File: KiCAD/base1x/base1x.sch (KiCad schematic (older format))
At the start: 82 parts, among them J1 Conn_02x05_Odd_Even, J10 Conn_01x03, J11 Conn_01x03, J12 Conn_01x03, J13 Conn_01x03, J14 Conn_01x03, J15 Conn_01x08, J17 Conn_01x03, J18 Conn_01x03, J19 Conn_01x03, J2 Conn_01x03, J3 Conn_02x14_Counter_Clockwise, J4 Conn_01x03, J5 Conn_01x03, J6 Conn_02x14_Counter_Clockwise, J7 Conn_02x06_Counter_Clockwise, J8 Conn_02x06_Counter_Clockwise, J9 Screw_Terminal_01x08, U2 ads122c04, U3 AD8615, U5 ads122c04, U6 AD8615, U7 AD8615, U8 LT1963AxQ-2.5, U9 LT3015xQ-2.5

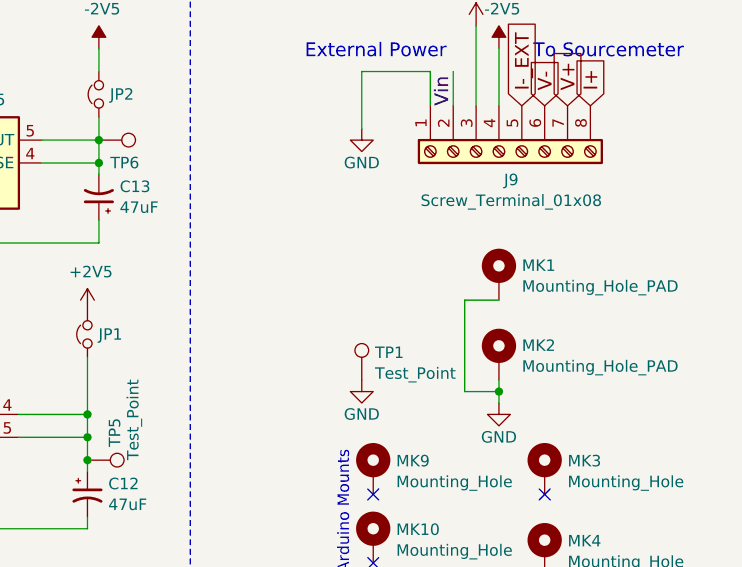
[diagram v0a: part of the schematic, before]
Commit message: work sync
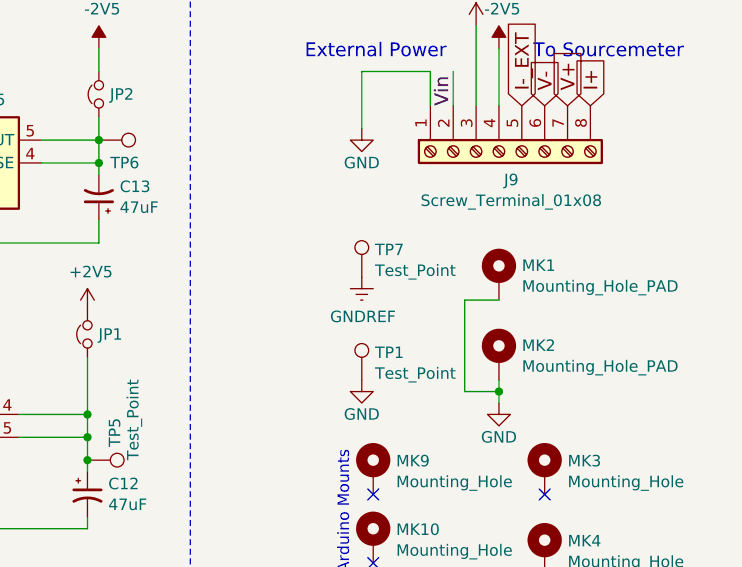
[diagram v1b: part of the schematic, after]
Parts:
- added TP7: Test_Point, myParts:Test_Point_S1751-46R, symbol Connector:TestPoint
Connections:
- net GNDREF: now also TP7.1
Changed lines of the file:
@@
 NoConn ~ 950  7400
 NoConn ~ 950  6900
+$Comp
+L Connector:TestPoint TP7
+U 1 1 5C3E8296
+P 9750 1850
+F 0 "TP7" H 9808 1970 50  0000 L CNN
+F 1 "Test_Point" H 9808 1879 50  0000 L CNN
+F 2 "myParts:Test_Point_S1751-46R" H 9950 1850 50  0001 C CNN
+F 3 "" H 9950 1850 50  0001 C CNN
+F 4 "2293786" H 4100 -4450 50  0001 C CNN "farnellCode"
+	1    9750 1850
+	1    0    0    -1
+$EndComp
+$Comp
+L power:GNDREF #PWR022
+U 1 1 5C3F39DD
+P 9750 1850
+F 0 "#PWR022" H 9750 1600 50  0001 C CNN
+F 1 "GNDREF" H 9755 1677 50  0000 C CNN
+F 2 "" H 9750 1850 50  0001 C CNN
+F 3 "" H 9750 1850 50  0001 C CNN
+	1    9750 1850
+	1    0    0    -1
+$EndComp
 $EndSCHEMATC

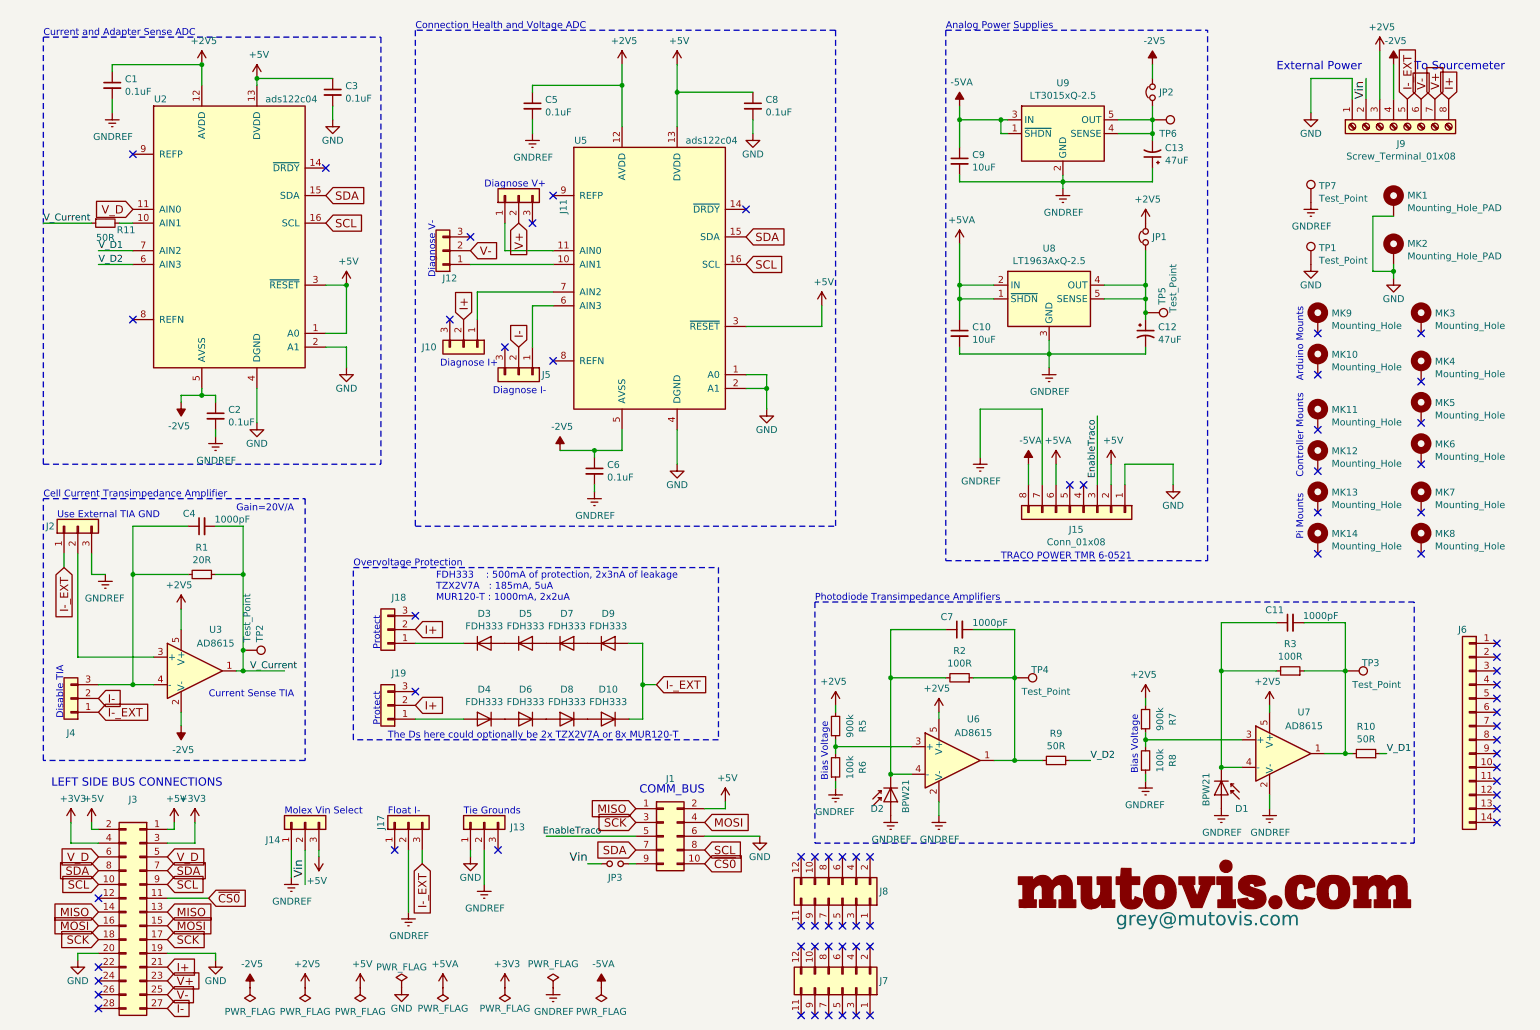
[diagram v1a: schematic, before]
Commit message: base1x doneish
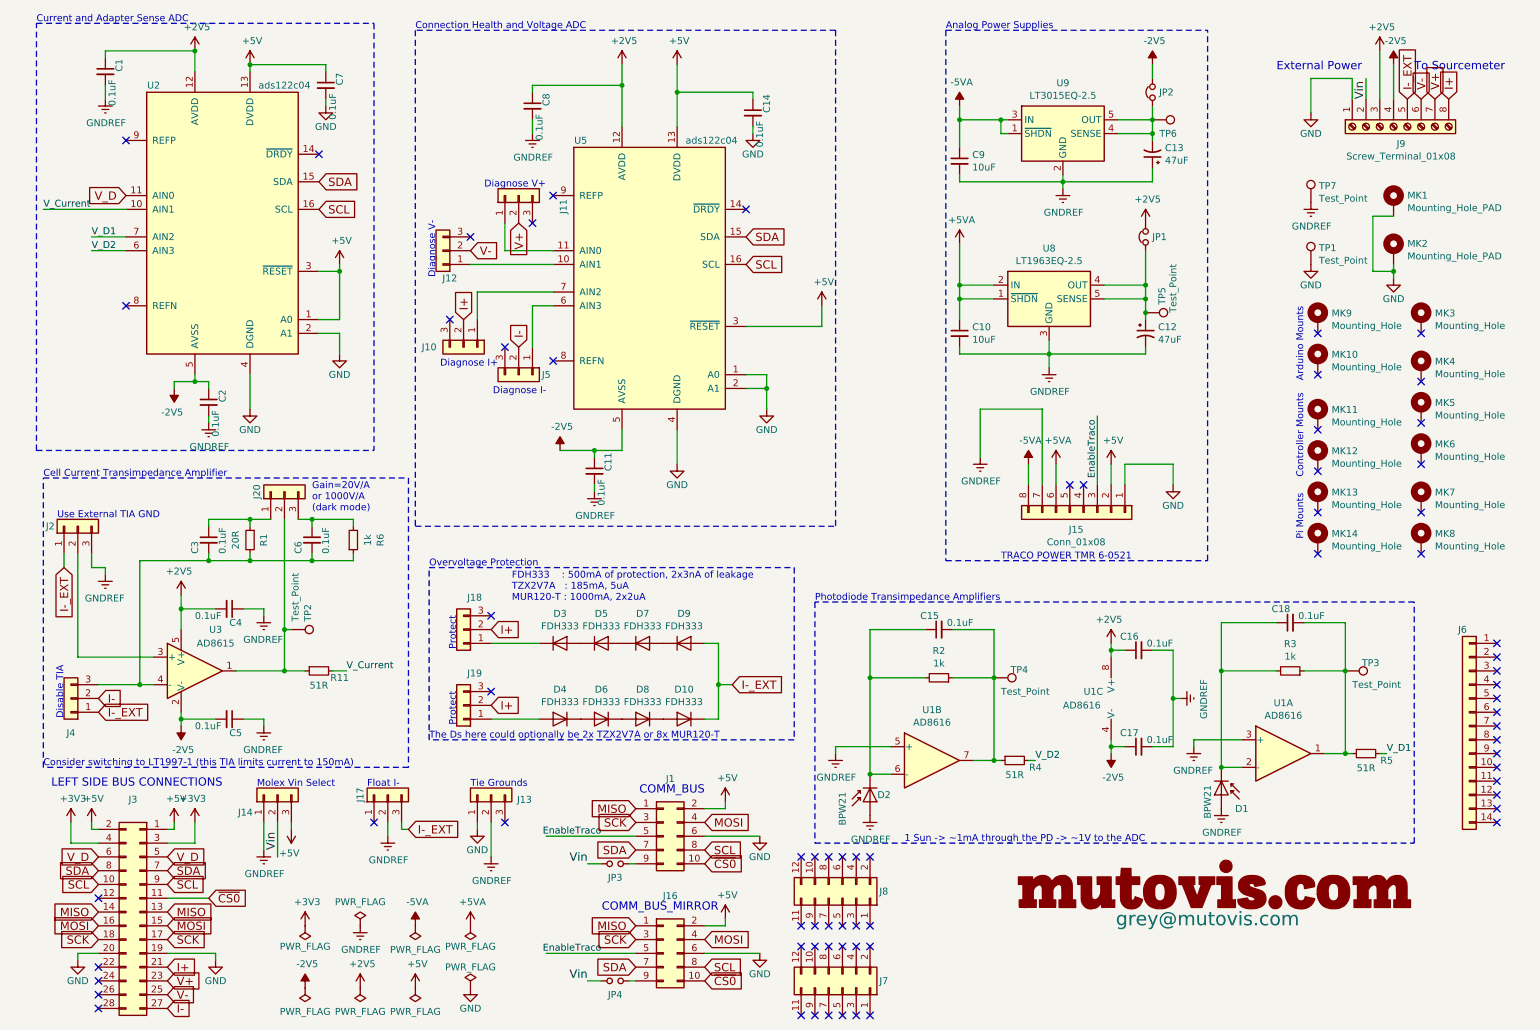
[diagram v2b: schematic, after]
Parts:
- removed R10, R9: 50R, Resistor_SMD:R_1206_3216Metric, symbol Device:R_Small
- removed R7: 900k, Resistor_SMD:R_1206_3216Metric, symbol Device:R_Small
- removed R8: 100k, Resistor_SMD:R_1206_3216Metric, symbol Device:R_Small
- removed U6, U7: AD8615, Package_TO_SOT_SMD:TSOT-23-5, symbol Amplifier_Operational:AD8603
- added C14, C15, C16, C17, C18: 0.1uF, Capacitor_SMD:C_1206_3216Metric, symbol Device:C_Small
- added J16: Conn_02x05_Odd_Even, Connector_IDC:IDC-Header_2x05_P2.54mm_Vertical, symbol Connector_Generic:Conn_02x05_Odd_Even
- added J20: Conn_01x03, Connector_PinHeader_1.27mm:PinHeader_1x03_P1.27mm_Vertical, symbol Connector_Generic:Conn_01x03
- added JP4: Jumper_NO_Small, Jumper:SolderJumper-2_P1.3mm_Open_RoundedPad1.0x1.5mm, symbol Device:Jumper_NO_Small
- added R4: 51R, Resistor_SMD:R_1206_3216Metric_Pad1.42x1.75mm_HandSolder, symbol Device:R_Small
- added U1: AD8616, Package_SO:SOIC-8_3.9x4.9mm_P1.27mm, symbol Amplifier_Operational:AD8620
- C1, C2, C3, C5, C6, C8: farnell code (none) -> 1759297
- C10, C9: farnell code (none) -> 1759453
- C11, C4, C7: value 1000pF -> 0.1uF; farnell code 1855909 -> 1759297
- C12, C13: footprint (none) -> Capacitor_Tantalum_SMD:CP_EIA-7343-43_Kemet-X_Pad2.25x2.55mm_HandSolder
- D1, D2: I_max 20mA -> 2mA
- D10, D3, D4, D5, D6, D7, D8, D9: farnellCode (none) -> 9843760
- J1: footprint Connector_IDC:IDC-Header_2x05_P2.54mm_Horizontal -> Connector_IDC:IDC-Header_2x05_P2.54mm_Vertical; farnellCode 2215290 -> 2215304
- J10, J11, J12, J13, J14, J17, J18, J19, J2, J4, J5: footprint (none) -> Connector_PinHeader_1.27mm:PinHeader_1x03_P1.27mm_Vertical; farnell code (none) -> 2578712+2505013
- J15: footprint (none) -> Converter_DCDC:Converter_DCDC_TRACO_TMR-xxxx_THT; Farnell Code (none) -> 495-TMR6-0521
- J3: farnell code (none) -> 1097986
- J6: value Conn_02x14_Counter_Clockwise -> Conn_01x14_Counter_Clockwise; footprint Connector_PinSocket_2.54mm:PinSocket_2x14_P2.54mm_Vertical -> Connector_PinHeader_2.54mm:PinHeader_1x14_P2.54mm_Vertical; farnellCode (none) -> 1593466
- JP3: footprint (none) -> Jumper:SolderJumper-2_P1.3mm_Open_RoundedPad1.0x1.5mm
- R1: footprint Resistor_SMD:R_1206_3216Metric -> Resistor_SMD:R_2010_5025Metric_Pad1.52x2.65mm_HandSolder; farnellCode 2073607 -> 1887405
- R11: value 50R -> 51R; footprint Resistor_SMD:R_1206_3216Metric -> Resistor_SMD:R_1206_3216Metric_Pad1.42x1.75mm_HandSolder; farnellCode 2476379 -> 2695165
- R2, R3: value 100R -> 1k; footprint Resistor_SMD:R_1206_3216Metric -> Resistor_SMD:R_1206_3216Metric_Pad1.42x1.75mm_HandSolder; farnellCode 2476379 -> 2447473
- R5: value 900k -> 51R; footprint Resistor_SMD:R_1206_3216Metric -> Resistor_SMD:R_1206_3216Metric_Pad1.42x1.75mm_HandSolder; farnellCode 2476379 -> 2695165
- R6: value 100k -> 1k; footprint Resistor_SMD:R_1206_3216Metric -> Resistor_SMD:R_1206_3216Metric_Pad1.42x1.75mm_HandSolder; farnellCode 2476379 -> 2447473
- U2, U5: footprint (none) -> Package_SO:TSSOP-16_4.4x5mm_P0.65mm; Farnell Code (none) -> 296-50885-1-ND
- U8: value LT1963AxQ-2.5 -> LT1963EQ-2.5; Farnell Code (none) -> LT1963EQ-2.5#PBF-ND
- U9: value LT3015xQ-2.5 -> LT3015EQ-2.5; Farnell Code (none) -> 584-LT3015EQ-2.5#PBF
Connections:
- net +2V5: now also C4.2, C8.1, C16.1, U1.8 (V+); no longer C5.1, R5.2
- net +5V: now also C7.1, C14.1, J16.2 (Pin_2); no longer C3.1, C8.1
- net -2V5: now also C11.1, C5.2, C17.1, U1.4 (V-); no longer C6.1
- net EnableTraco: now also J16.5 (Pin_5)
- net GND: now also C7.2, C14.2, J16.6 (Pin_6); no longer C3.2, C8.2
- net GNDREF: now also C11.2, C4.1, C5.1, C8.2, C16.2, C17.2, U1.3 (+), U1.5 (+); no longer C5.2, C6.2, R6.1
- net MISO: now also J16.1 (Pin_1)
- net MOSI: now also J16.4 (Pin_4)
- net SCK: now also J16.3 (Pin_3)
- net SCL: now also J16.8 (Pin_8)
- net SDA: now also J16.7 (Pin_7)
- net V_Current: now also R11.2, U2.10 (AIN1); no longer C4.2, R1.1, R11.1, TP2.1, U3.1
- net V_D1: now also R5.2
- net V_D2: now also R4.2
- net Vin: now also JP4.1
- net ~CS0: now also J16.10 (Pin_10)
- net at D1.1 (K), R3.2: now also C18.1, U1.2 (-); no longer C11.1
- net at D2.1 (K), R2.2: now also C15.1, U1.6 (-); no longer C7.1
- net at R2.1, TP4.1: now also C15.2, R4.1, U1.7; no longer C7.2
- net at R5.1: now also R3.1, TP3.1, C18.2, U1.1; no longer R6.2
- net at J4.3 (Pin_3), R1.2, U3.4 (-): now also C3.2, C6.2, R6.1; no longer C4.1
- new net: J16.9 (Pin_9), JP4.2
- new net: J20.2 (Pin_2), R11.1, TP2.1, U3.1
- new net: C3.1, J20.1 (Pin_1), R1.1
- new net: C6.1, J20.3 (Pin_3), R6.2
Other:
- note added: "1 Sun -> ~~1mA through the PD -> ~~1V to the ADC"
- note added: "COMM_BUS_MIRROR"
- note added: "Consider switching to LT1997-1 (this TIA limits current to 150mA)"
- note added: "Gain=20V/A\nor 1000V/A\n(dark mode)"
- note removed: "Bias Voltage"
- note removed: "Current Sense TIA"
- note removed: "Gain=20V/A"
- moved on the sheet: D10, D2, D3, D4, D5, D6, D7, D8, D9, J13, J14, J17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
